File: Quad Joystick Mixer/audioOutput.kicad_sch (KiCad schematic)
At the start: 26 parts, among them J2 NMJ6HCD, U4 TL072

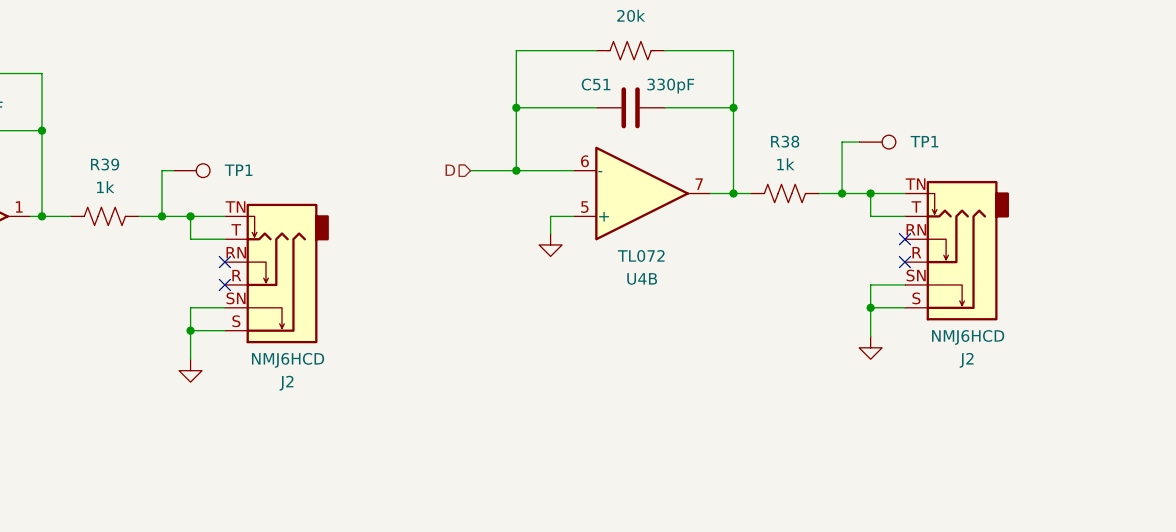
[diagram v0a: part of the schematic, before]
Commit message: major layout progress
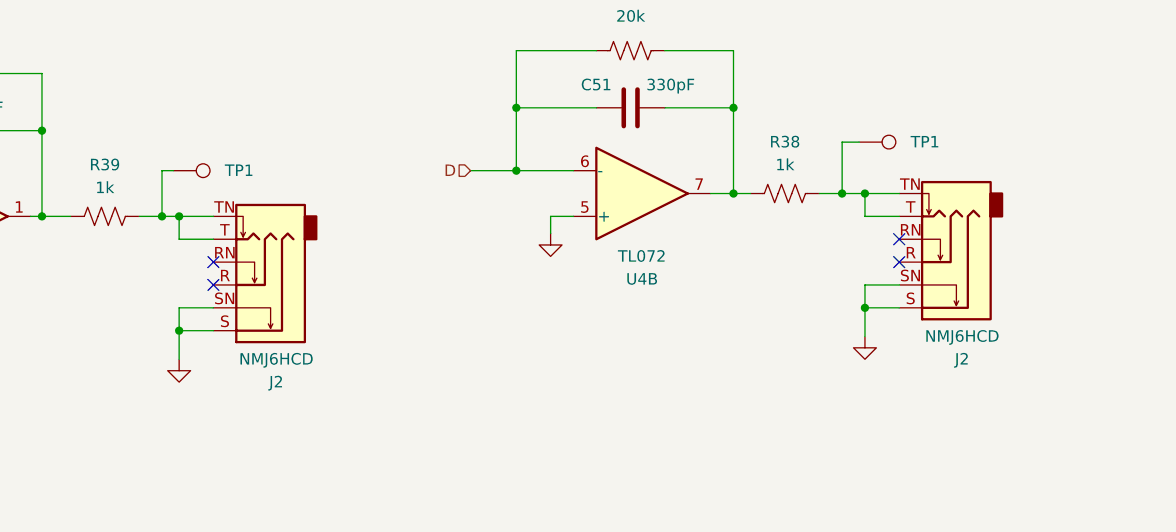
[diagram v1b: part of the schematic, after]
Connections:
- net at R38.1, TP1.1: now also J2.T, J2.TN; no longer J2.T, J2.TN
- net at R39.1, TP1.1: now also J2.T, J2.TN; no longer J2.T, J2.TN
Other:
- moved on the sheet: J2
